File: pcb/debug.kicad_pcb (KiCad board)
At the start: 2 copper layers, 65 parts, among them J1 09732966801, J2 USB_C_Receptacle_USB2.0, Q1 Q_PNP_BCE, SW1 SW_DIP_x02, SW2 Reset, U1 STLQ020PU33R, U2 FT4222HQ, U3 STM32F103V8Tx, U4 INA381AxDSG, U5 SN74ALVC00, U6 MIC94090, Y1 12MHz, Y2 24MHz

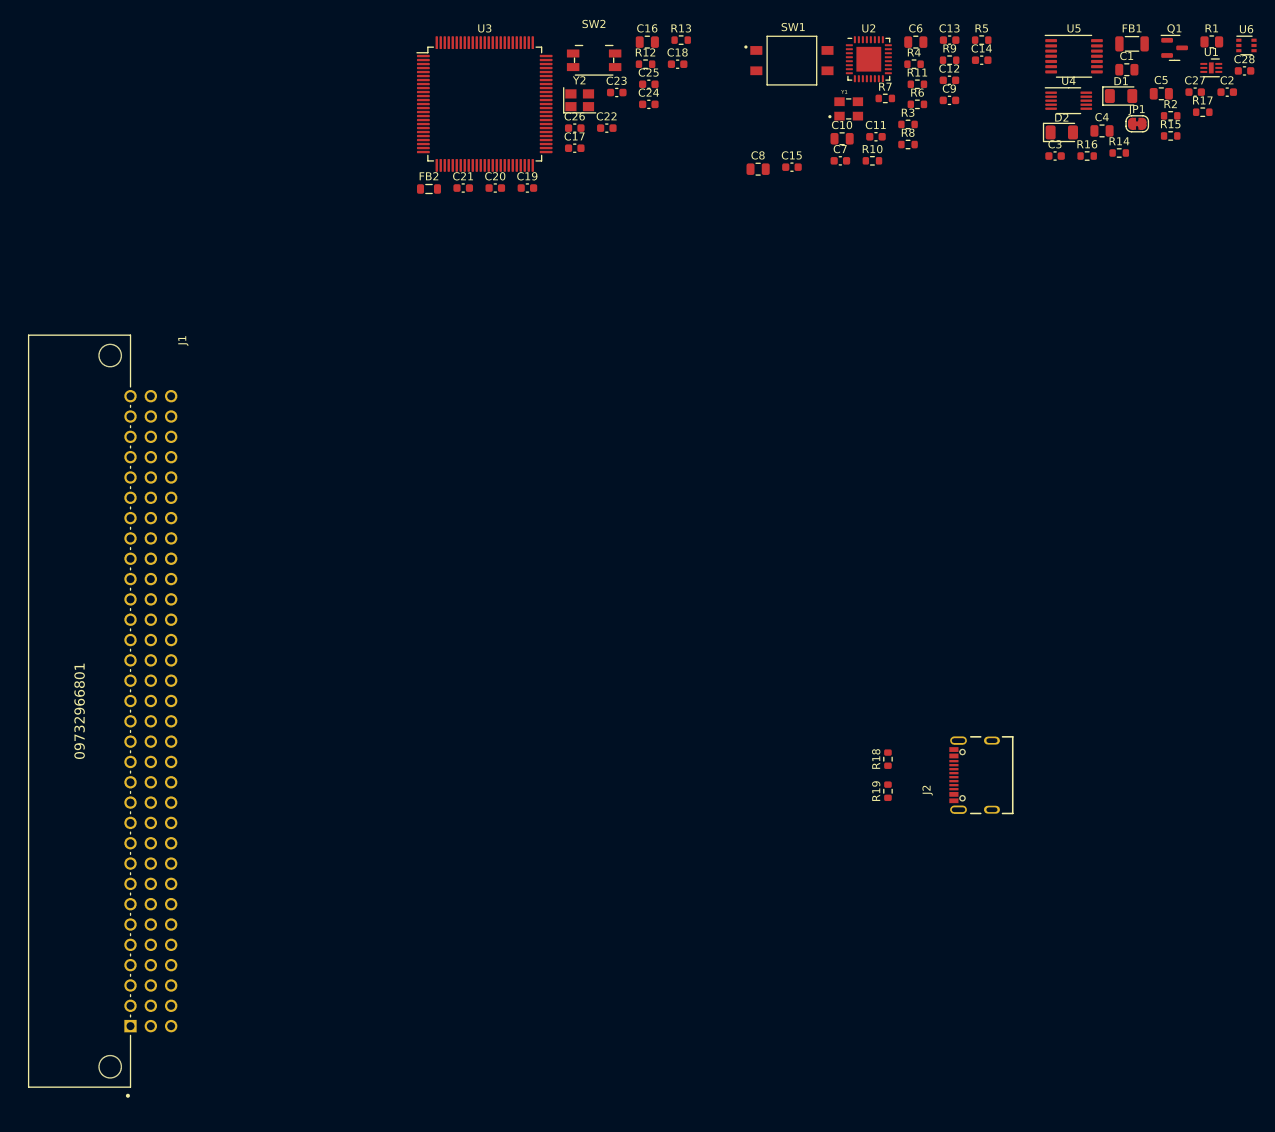
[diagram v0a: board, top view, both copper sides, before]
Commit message: start placing components
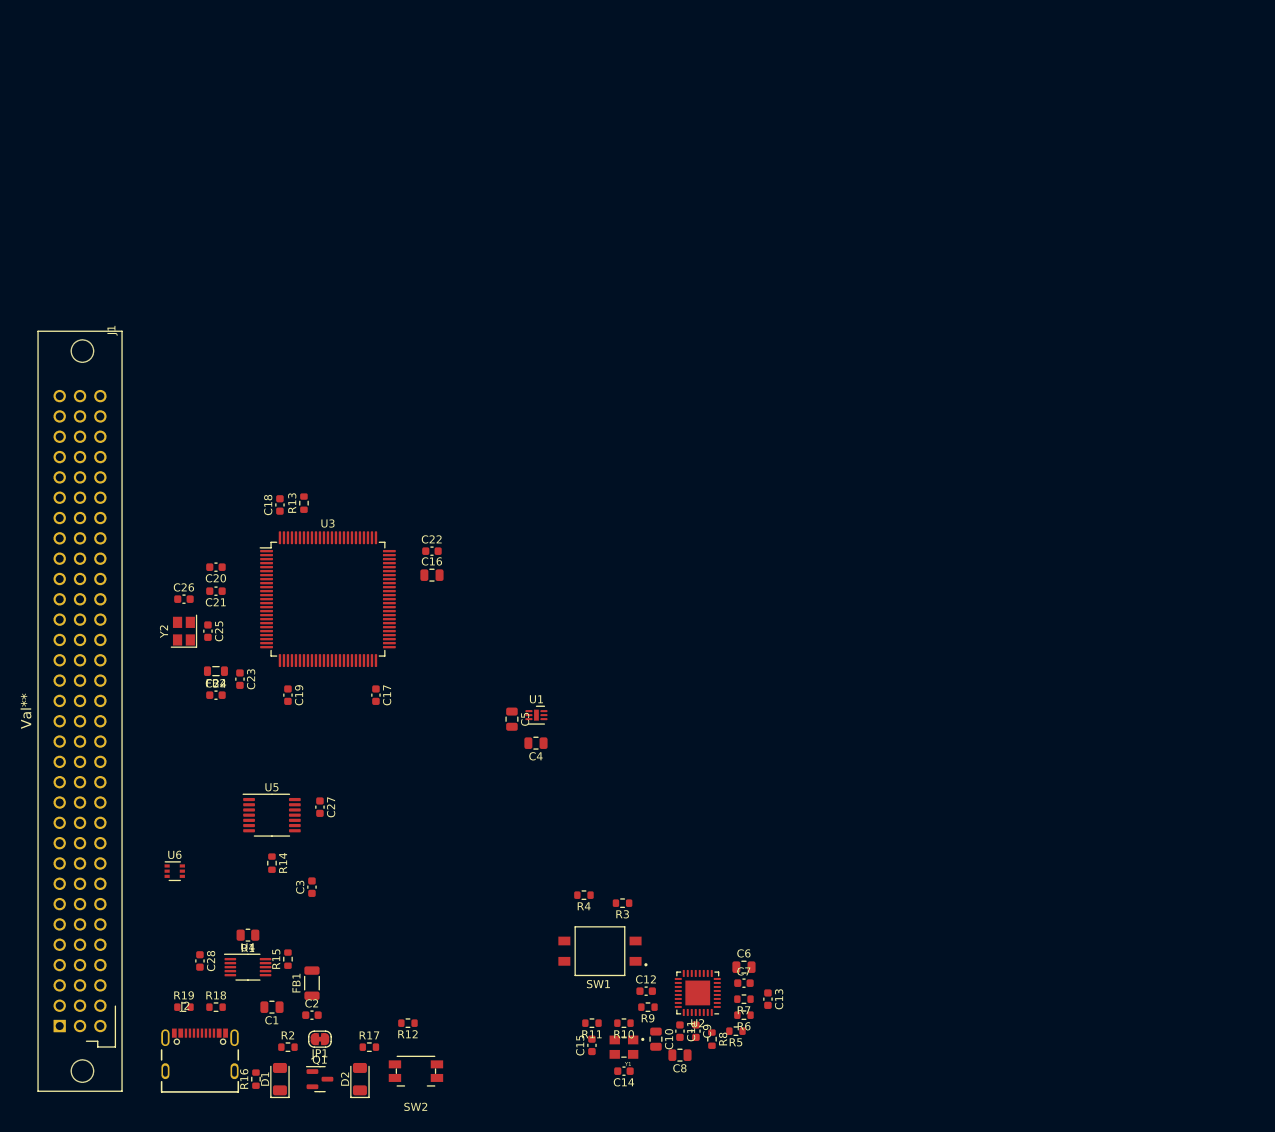
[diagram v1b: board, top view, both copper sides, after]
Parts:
- J1: value 09732966801 -> Val**; footprint 09031966821:Harting-09031966921-0-0-0 -> 09031966821:09032967825
- moved C28 171.5 mm to (101.0, 129.2), turned to -90 degrees
- moved U6 169.1 mm to (97.8, 118.0)
- moved Q1 167.4 mm to (116.0, 144.0)
- moved R1 164.3 mm to (107.0, 126.0), turned to 180 degrees
- moved C2 162.5 mm to (115.0, 136.0)
- moved D1 161.7 mm to (111.0, 144.0), turned to 90 degrees
- moved R2 160.4 mm to (112.0, 140.0)
- moved C1 158.6 mm to (110.0, 135.0), turned to 180 degrees
- moved R17 156.6 mm to (122.2, 140.0)
- moved FB1 155.9 mm to (115.0, 132.0), turned to 90 degrees
- moved R16 155.3 mm to (108.0, 144.0), turned to 90 degrees
- moved JP1 153.4 mm to (116.0, 139.0), turned to 180 degrees
- moved R15 150.9 mm to (112.0, 129.0), turned to 90 degrees
- moved U4 149.2 mm to (107.0, 130.0)
- moved D2 147.3 mm to (121.0, 144.0), turned to 90 degrees
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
